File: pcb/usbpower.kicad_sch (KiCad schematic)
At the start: 13 parts, among them J1 USB_C_Receptacle_USB2.0_16P, Q1 AO3401A, U1 SPX3819M5-L-3-3

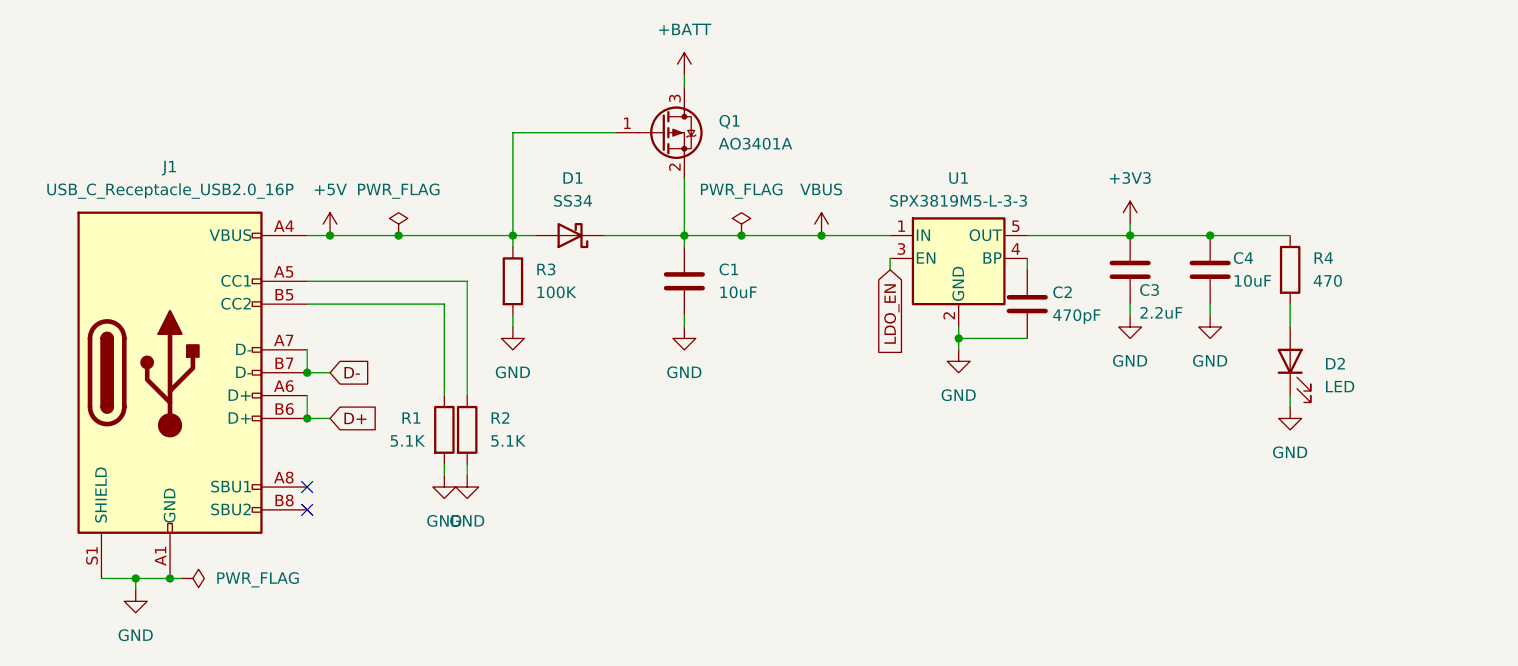
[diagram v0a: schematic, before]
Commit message: with errors
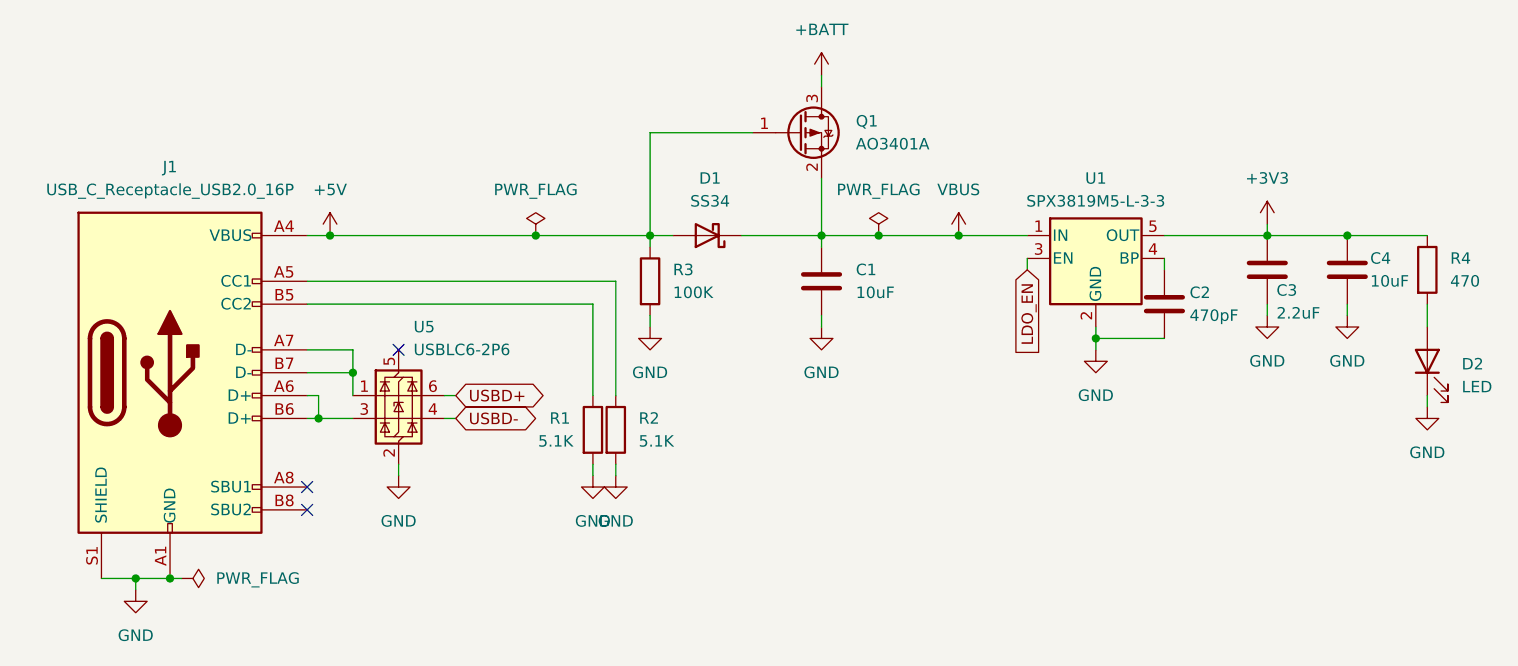
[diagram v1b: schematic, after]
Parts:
- added U5: USBLC6-2P6, Package_TO_SOT_SMD:SOT-666, symbol Power_Protection:USBLC6-2P6
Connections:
- net GND: now also U5.2 (GND)
- net D+: no longer names the net of J1.A6 (D+), J1.B6 (D+)
- net D+: now also U5.3 (I/O2)
- net D-: no longer names the net of J1.A7 (D-), J1.B7 (D-)
- net D-: now also U5.1 (I/O1)
- new net USBD+: U5.6 (I/O1)
- new net USBD-: U5.4 (I/O2)
- no-connect marks 2 -> 3
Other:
- moved on the sheet: C1, C2, C3, C4, D1, D2, Q1, R1, R2, R3, R4, U1
